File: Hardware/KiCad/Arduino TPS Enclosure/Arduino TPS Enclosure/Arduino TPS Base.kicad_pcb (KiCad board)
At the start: 2 copper layers, 73.7 x 94 mm, 3 parts

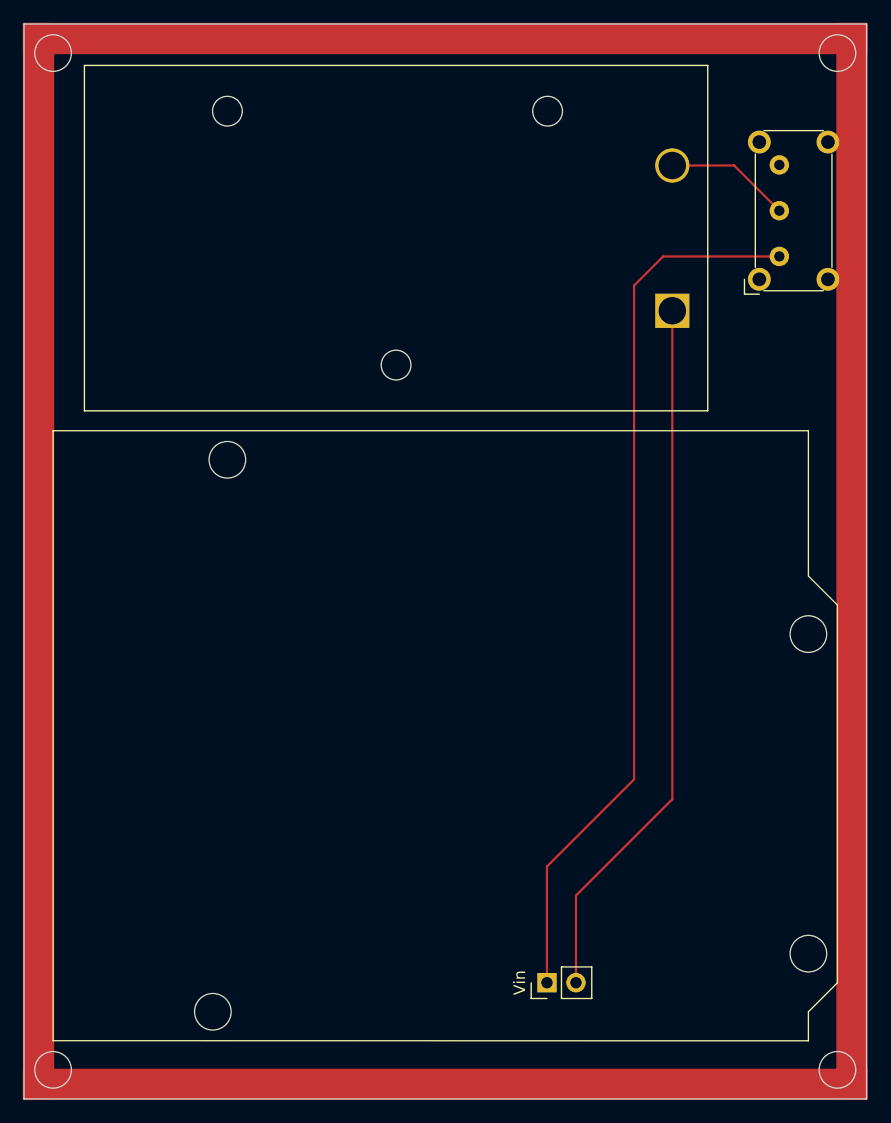
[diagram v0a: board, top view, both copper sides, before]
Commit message: Update
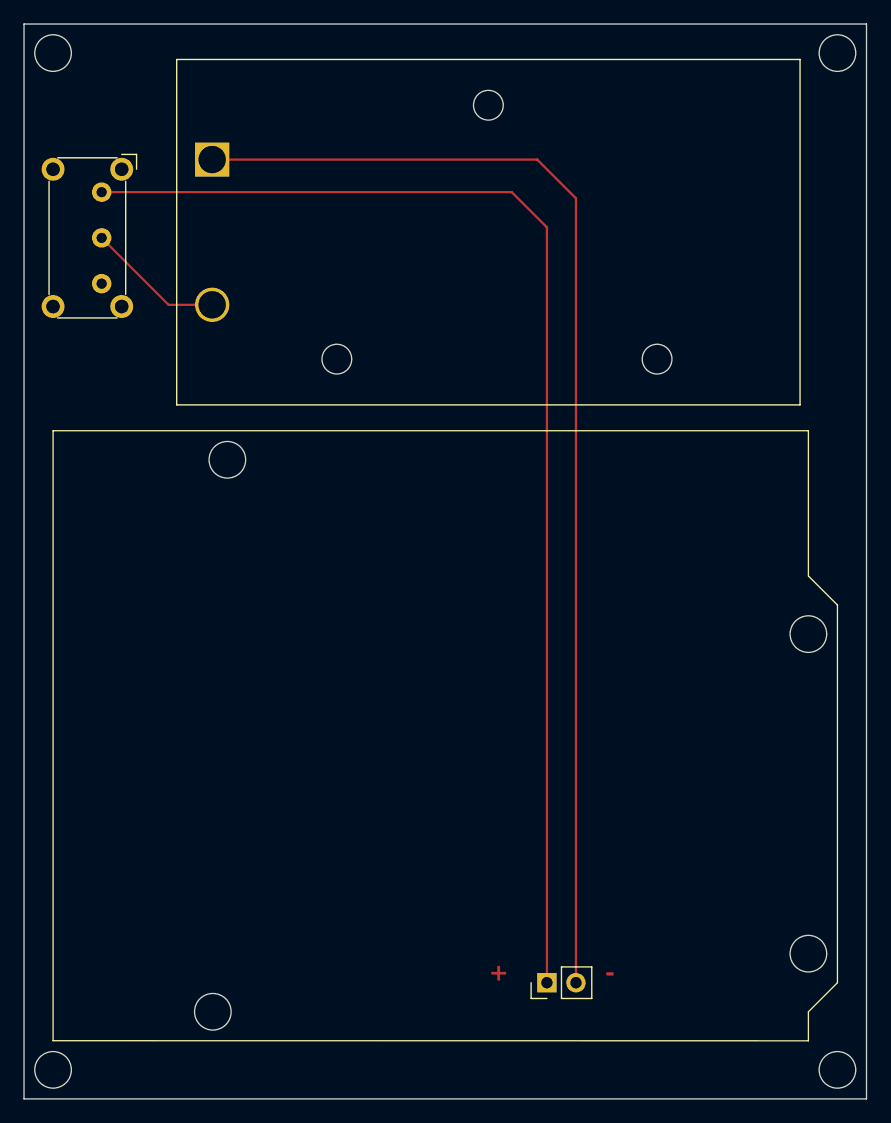
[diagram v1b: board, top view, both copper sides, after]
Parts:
- moved REF** 59.5 mm to (32.2, 40.1), turned to -90 degrees
- moved REF** 42.3 mm to (41.9, 37.2), turned to 180 degrees
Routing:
- net (no net): track 151.1 -> 220.1 mm
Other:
- board text added: "+"
- board text added: "-"
